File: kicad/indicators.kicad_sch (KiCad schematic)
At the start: 36 parts, among them J9 Free pin, U14 74LS244

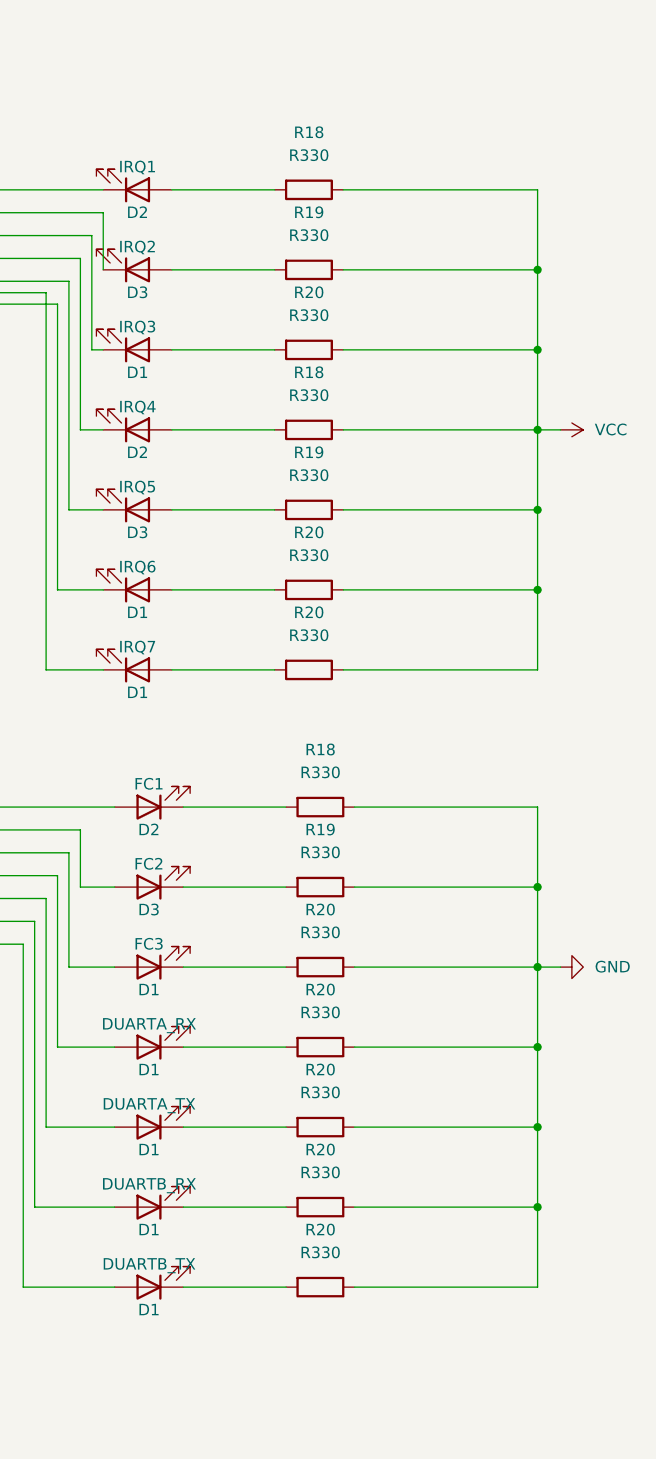
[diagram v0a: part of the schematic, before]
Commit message: got irq to work
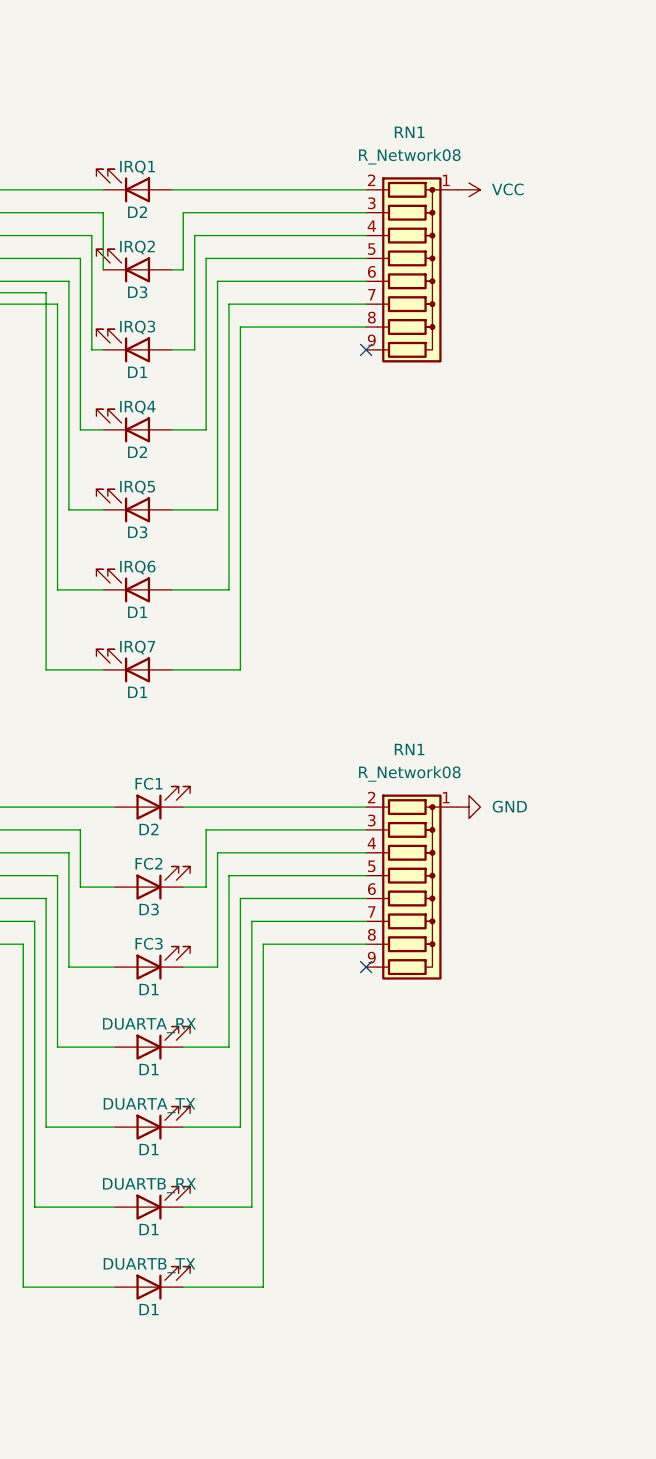
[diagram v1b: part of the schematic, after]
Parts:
- removed R18 (x3), R19 (x3), R20 (x8): R330, Resistor_THT:R_Axial_DIN0207_L6.3mm_D2.5mm_P10.16mm_Horizontal, symbol Device:R
- added RN1 (x2): R_Network08, Resistor_THT:R_Array_SIP9, symbol Device:R_Network08
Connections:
- net GND: now also RN1.1 (common)
- net VCC: now also RN1.1 (common)
- net at D3.2 (A): now also RN1.3 (R2)
- net at D1.1 (K): now also RN1.5 (R4)
- net at D2.2 (A): now also RN1.5 (R4)
- net at D2.2 (A): now also RN1.2 (R1)
- net at D3.1 (K): now also RN1.3 (R2)
- net at D1.1 (K): now also RN1.4 (R3)
- net at D1.1 (K): now also RN1.8 (R7)
- net at D1.1 (K): now also RN1.6 (R5)
- net at D1.2 (A): now also RN1.4 (R3)
- net at D1.2 (A): now also RN1.7 (R6)
- net at D2.1 (K): now also RN1.2 (R1)
- net at D1.1 (K): now also RN1.7 (R6)
- net at D1.2 (A): now also RN1.8 (R7)
- net at D3.2 (A): now also RN1.6 (R5)
- no-connect marks 0 -> 2
